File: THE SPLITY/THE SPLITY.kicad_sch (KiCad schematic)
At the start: 59 parts, among them U2 Nice_Nano_V2

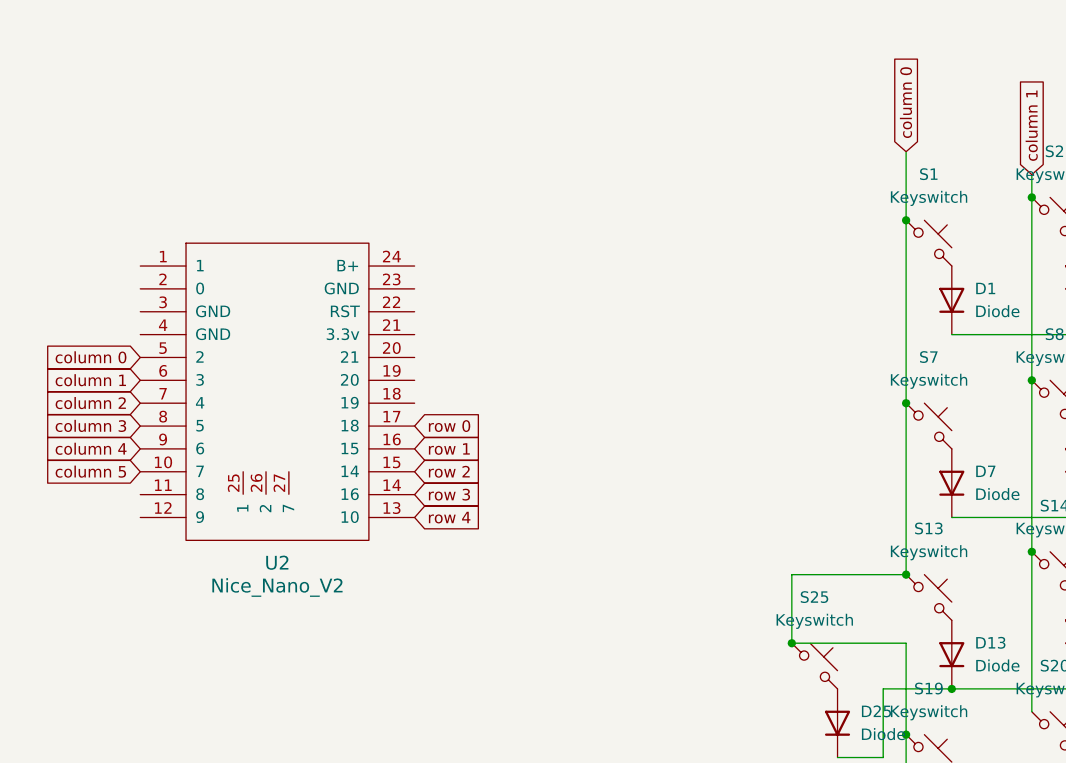
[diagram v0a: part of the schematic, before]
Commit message: added a battery connector
boo
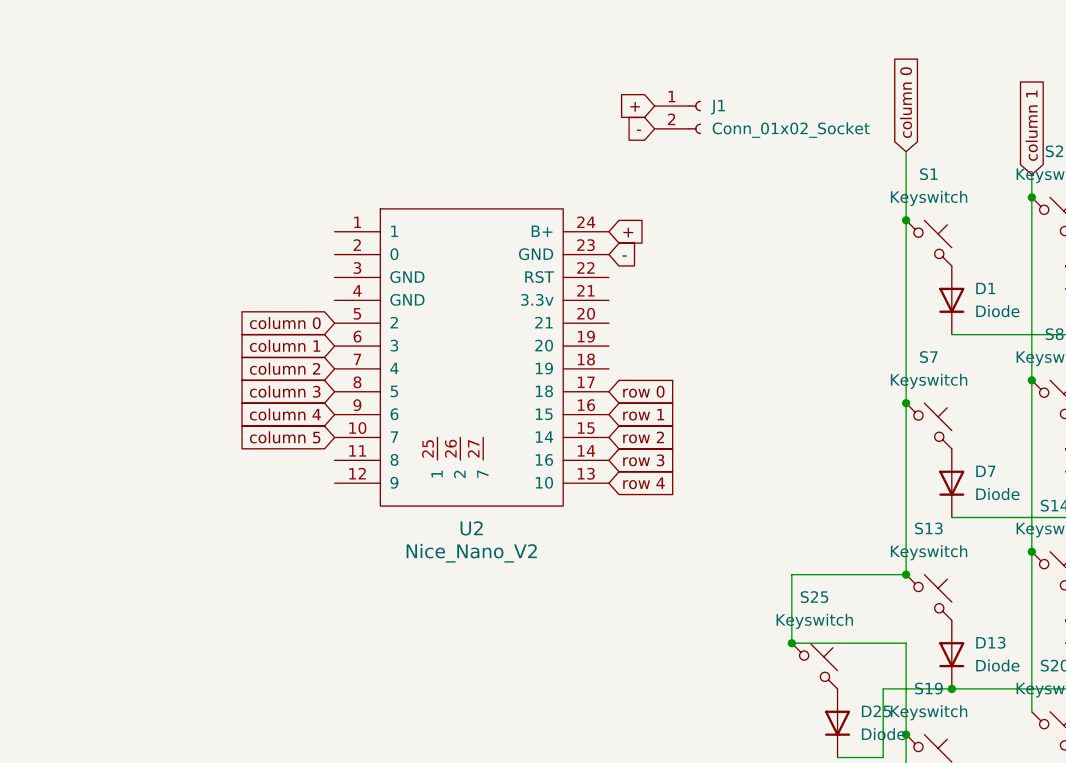
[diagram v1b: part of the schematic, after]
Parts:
- added J1: Conn_01x02_Socket, Connector_JST:JST_XH_B2B-XH-AM_1x02_P2.50mm_Vertical, symbol Connector:Conn_01x02_Socket
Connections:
- net -: now reaches U2.23 (GND)
- net -: now also J1.2 (Pin_2)
- net +: now reaches U2.24 (B+)
- net +: now also J1.1 (Pin_1)
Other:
- moved on the sheet: U2
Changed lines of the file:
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@@
 	(global_label "column 5"
 		(shape input)
-		(at 57.15 114.3 180)
+		(at 78.74 110.49 180)
 		(fields_autoplaced yes)
 		(effects
@@
 		)
 		(property "Intersheetrefs" "${INTERSHEET_REFS}"
-			(at 45.0936 114.3 0)
+			(at 66.6836 110.49 0)
 			(effects
 				(font
@@
 	(global_label "row 0"
 		(shape input)
-		(at 87.63 109.22 0)
+		(at 109.22 105.41 0)
 		(fields_autoplaced yes)
 		(effects
@@
 		)
 		(property "Intersheetrefs" "${INTERSHEET_REFS}"
-			(at 96.058 109.22 0)
+			(at 117.648 105.41 0)
 			(effects
 				(font
@@
 	(global_label "column 3"
 		(shape input)
-		(at 57.15 109.22 180)
+		(at 78.74 105.41 180)
 		(fields_autoplaced yes)
 		(effects
@@
 		)
 		(property "Intersheetrefs" "${INTERSHEET_REFS}"
-			(at 45.0936 109.22 0)
+			(at 66.6836 105.41 0)
 			(effects
 				(font
@@
 	(global_label "column 4"
 		(shape input)
-		(at 57.15 111.76 180)
+		(at 78.74 107.95 180)
 		(fields_autoplaced yes)
 		(effects
@@
 		)
 		(property "Intersheetrefs" "${INTERSHEET_REFS}"
-			(at 45.0936 111.76 0)
+			(at 66.6836 107.95 0)
 			(effects
 				(font
@@
 		)
 	)
+	(global_label "-"
+		(shape input)
+		(at 109.22 90.17 0)
+		(fields_autoplaced yes)
+		(effects
+			(font
+				(size 1.27 1.27)
+			)
+			(justify left)
+		)
+		(property "Intersheetrefs" "${INTERSHEET_REFS}"
+			(at 113.7776 90.17 0)
+			(effects
+				(font
+					(size 1.27 1.27)
+				)
+				(justify left)
+				(hide yes)
+			)
+		)
+	)
 	(global_label "column 1"
 		(shape input)
-		(at 57.15 104.14 180)
+		(at 78.74 100.33 180)
+		(fields_autoplaced yes)
+		(effects
+			(font
+				(size 1.27 1.27)
+			)
+			(justify right)
+		)
+		(property "Intersheetrefs" "${INTERSHEET_REFS}"
+			(at 66.6836 100.33 0)
+			(effects
+				(font
+					(size 1.27 1.27)
+				)
+				(justify right)
+				(hide yes)
+			)
+		)
+	)
+	(global_label "-"
+		(shape input)
+		(at 114.3 76.2 180)
 		(fields_autoplaced yes)
 		(effects
@@
 		)
 		(property "Intersheetrefs" "${INTERSHEET_REFS}"
-			(at 45.0936 104.14 0)
+			(at 109.7424 76.2 0)
 			(effects
 				(font
@@
 	(global_label "row 3"
 		(shape input)
-		(at 87.63 116.84 0)
+		(at 109.22 113.03 0)
 		(fields_autoplaced yes)
 		(effects
@@
 		)
 		(property "Intersheetrefs" "${INTERSHEET_REFS}"
-			(at 96.058 116.84 0)
+			(at 117.648 113.03 0)
 			(effects
 				(font
@@
 		)
 	)
+	(global_label "+"
+		(shape input)
+		(at 114.3 73.66 180)
+		(fields_autoplaced yes)
+		(effects
+			(font
+				(size 1.27 1.27)
+			)
+			(justify right)
+		)
+		(property "Intersheetrefs" "${INTERSHEET_REFS}"
+			(at 109.7424 73.66 0)
+			(effects
+				(font
+					(size 1.27 1.27)
+				)
+				(justify right)
+				(hide yes)
+			)
+		)
+	)
 	(global_label "column 0"
 		(shape input)
@@
 	(global_label "row 1"
 		(shape input)
-		(at 87.63 111.76 0)
+		(at 109.22 107.95 0)
 		(fields_autoplaced yes)
 		(effects
@@
 		)
 		(property "Intersheetrefs" "${INTERSHEET_REFS}"
-			(at 96.058 111.76 0)
+			(at 117.648 107.95 0)
+			(effects
+				(font
+					(size 1.27 1.27)
+				)
+				(justify left)
+				(hide yes)
+			)
+		)
+	)
+	(global_label "+"
+		(shape input)
+		(at 109.22 87.63 0)
+		(fields_autoplaced yes)
+		(effects
+			(font
+				(size 1.27 1.27)
+			)
+			(justify left)
+		)
+		(property "Intersheetrefs" "${INTERSHEET_REFS}"
+			(at 113.7776 87.63 0)
 			(effects
 				(font
@@
 	(global_label "row 2"
 		(shape input)
-		(at 87.63 114.3 0)
+		(at 109.22 110.49 0)
 		(fields_autoplaced yes)
 		(effects
@@
 		)
 		(property "Intersheetrefs" "${INTERSHEET_REFS}"
-			(at 96.058 114.3 0)
+			(at 117.648 110.49 0)
 			(effects
 				(font
@@
 	(global_label "column 2"
 		(shape input)
-		(at 57.15 106.68 180)
+		(at 78.74 102.87 180)
 		(fields_autoplaced yes)
 		(effects
@@
 		)
 		(property "Intersheetrefs" "${INTERSHEET_REFS}"
-			(at 45.0936 106.68 0)
+			(at 66.6836 102.87 0)
 			(effects
 				(font
@@
 	(global_label "row 4"
 		(shape input)
-		(at 87.63 119.38 0)
+		(at 109.22 115.57 0)
 		(fields_autoplaced yes)
 		(effects
@@
 		)
 		(property "Intersheetrefs" "${INTERSHEET_REFS}"
-			(at 96.058 119.38 0)
+			(at 117.648 115.57 0)
 			(effects
 				(font
@@
 	(global_label "column 0"
 		(shape input)
-		(at 57.15 101.6 180)
+		(at 78.74 97.79 180)
 		(fields_autoplaced yes)
 		(effects
@@
 		)
 		(property "Intersheetrefs" "${INTERSHEET_REFS}"
-			(at 45.0936 101.6 0)
+			(at 66.6836 97.79 0)
 			(effects
 				(font
@@
 	(symbol
 		(lib_id "ScottoKeebs:MCU_Nice_Nano_V2")
-		(at 72.39 105.41 0)
+		(at 93.98 101.6 0)
 		(unit 1)
 		(exclude_from_sim no)
@@
 		(dnp no)
 		(property "Reference" "U2"
-			(at 72.39 124.46 0)
+			(at 93.98 120.65 0)
 			(effects
 				(font
@@
 		)
 		(property "Value" "Nice_Nano_V2"
-			(at 72.39 127 0)
+			(at 93.98 123.19 0)
 			(effects
 				(font
@@
 		)
 		(property "Footprint" "ScottoKeebs_MCU:Nice_Nano_V2_Flipped"
-			(at 72.39 128.27 0)
+			(at 93.98 124.46 0)
 			(effects
 				(font
@@
 		)
 		(property "Datasheet" ""
-			(at 99.06 168.91 90)
+			(at 120.65 165.1 90)
 			(effects
 				(font
@@
 		)
 		(property "Description" ""
-			(at 72.39 105.41 0)
+			(at 93.98 101.6 0)
 			(effects
 				(font
@@
 					(unit 1)
 				)
+			)
+		)
+	)
+	(symbol
+		(lib_id "Connector:Conn_01x02_Socket")
+		(at 119.38 73.66 0)
+		(unit 1)
+		(exclude_from_sim no)
+		(in_bom yes)
+		(on_board yes)
+		(dnp no)
+		(fields_autoplaced yes)
+		(property "Reference" "J1"
+			(at 120.65 73.6599 0)
+			(effects
+				(font
+					(size 1.27 1.27)
+				)
+				(justify left)
+			)
+		)
+		(property "Value" "Conn_01x02_Socket"
+			(at 120.65 76.1999 0)
+			(effects
+				(font
+					(size 1.27 1.27)
+				)
+				(justify left)
+			)
+		)
+		(property "Footprint" "Connector_JST:JST_XH_B2B-XH-AM_1x02_P2.50mm_Vertical"
+			(at 119.38 73.66 0)
+			(effects
+				(font
+					(size 1.27 1.27)
+				)
+				(hide yes)
+			)
+		)
+		(property "Datasheet" "~"
+			(at 119.38 73.66 0)
+			(effects
+				(font
+					(size 1.27 1.27)
+				)
+				(hide yes)
+			)
+		)
+		(property "Description" "Generic connector, single row, 01x02, script generated"
+			(at 119.38 73.66 0)
+			(effects
+				(font
+					(size 1.27 1.27)
+				)
+				(hide yes)
+			)
+		)
+		(pin "1"
+		)
+		(pin "2"
+		)
+		(instances
+			(project ""
+				(path "/d377bd6e-6f97-4d3e-8a43-76ce85113ab3"
+					(reference "J1")
+					(unit 1)
+				)

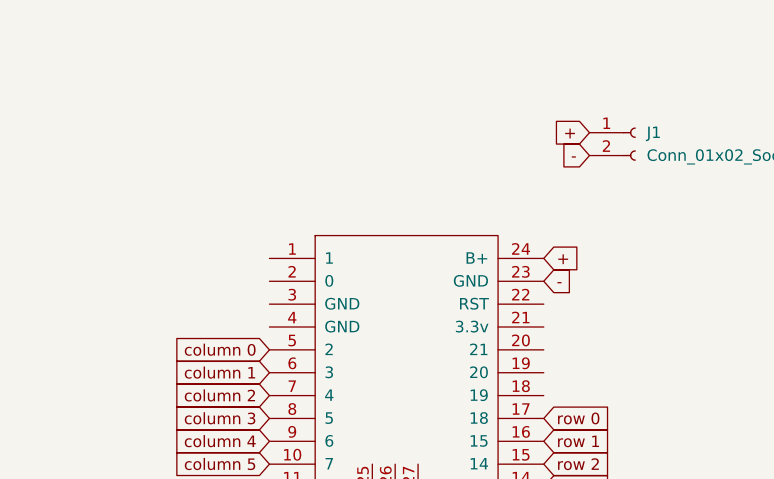
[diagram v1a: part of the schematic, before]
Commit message: ז
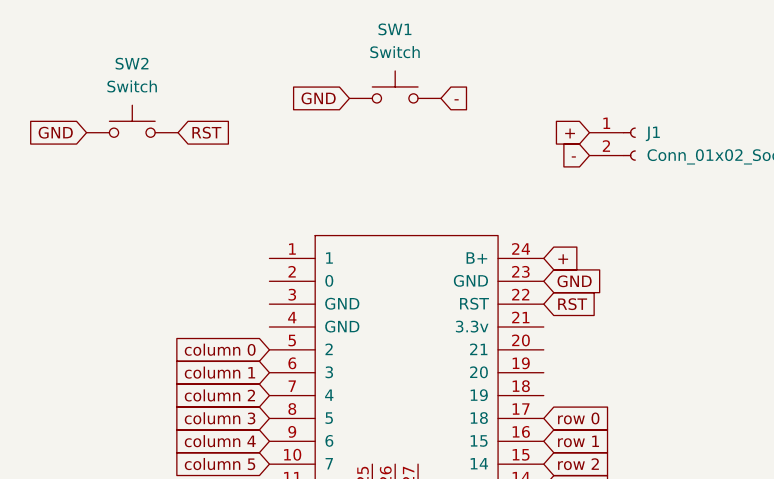
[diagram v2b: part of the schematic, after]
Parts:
- added SW1, SW2: Switch, symbol ScottoKeebs:Placeholder_Switch
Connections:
- net -: now also SW1.2; no longer U2.23 (GND)
- net RST: now reaches U2.22 (RST)
- net RST: now also SW2.2
- new net GND: SW1.1, SW2.1, U2.23 (GND)
